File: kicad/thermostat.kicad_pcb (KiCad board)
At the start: 2 copper layers, 65 x 56 mm, 11 parts, among them P1 Conn_02x20_Odd_Even, U1 RELAY_HEAT

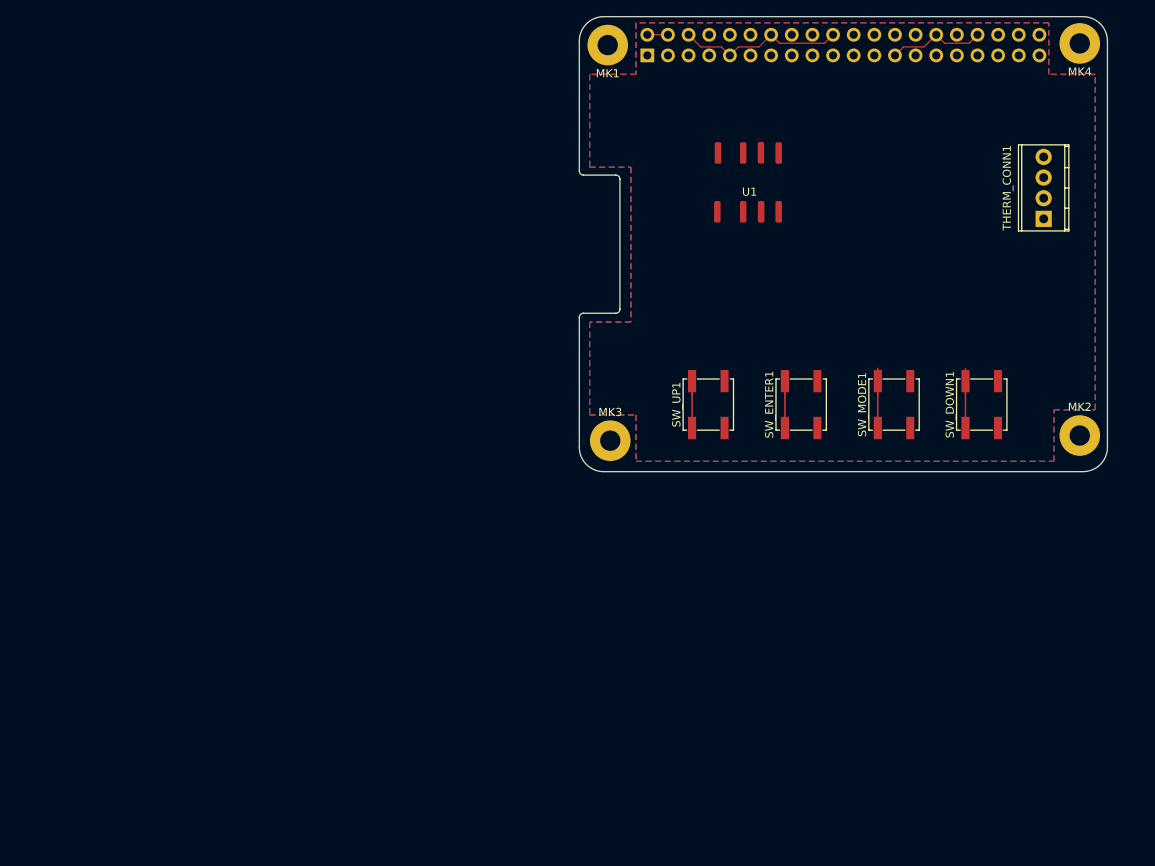
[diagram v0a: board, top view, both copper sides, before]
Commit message: First take at the bigger board
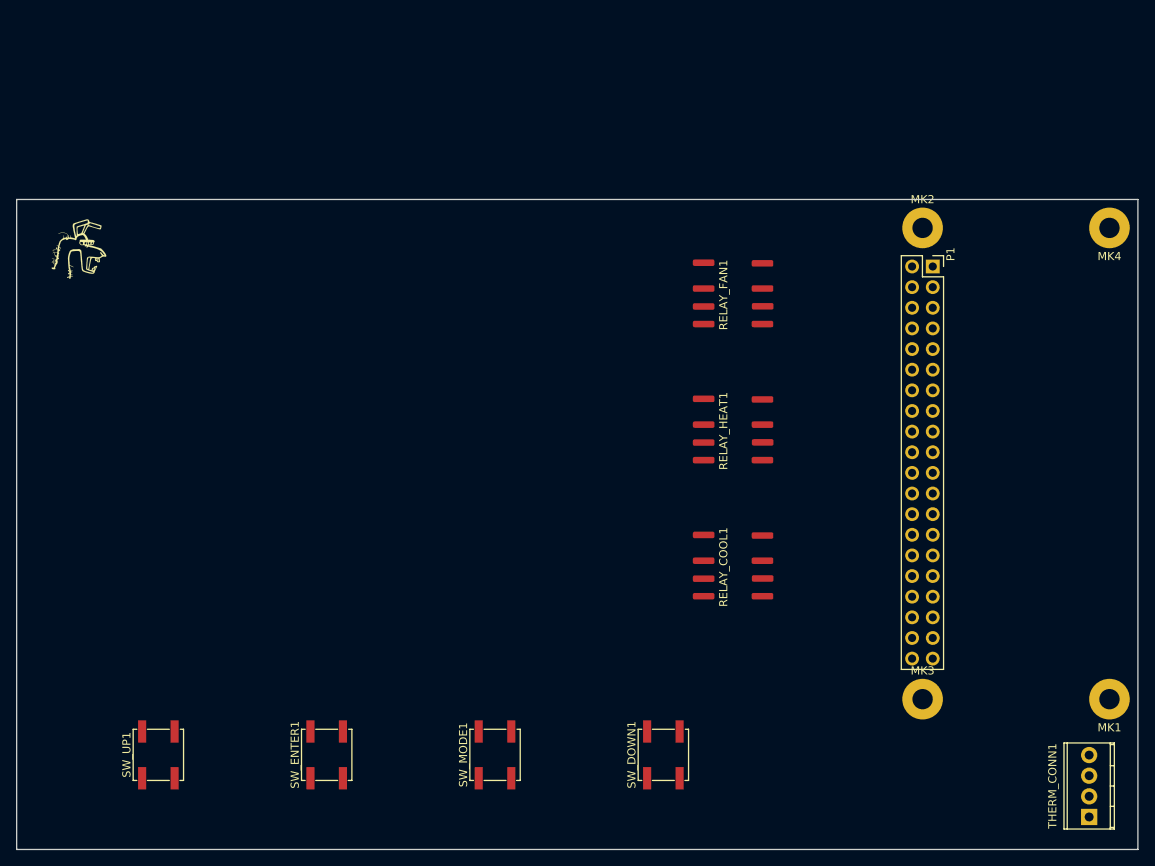
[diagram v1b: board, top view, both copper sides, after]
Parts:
- added G***: LOGO, project_footprints:LlamaHead, F.Cu at (138.5, 122.5)
- added RELAY_COOL1: RELAY_COOL, project_footprints:AGQ210A03, F.Cu at (218.2, 161.8)
- added RELAY_HEAT1: RELAY_HEAT, project_footprints:AGQ210A03, F.Cu at (218.2, 145.0)
- P1: moved to F.Cu
- RELAY_FAN1: renamed from U1; value RELAY_HEAT -> RELAY_FAN
- moved MK1 101.5 mm to (265.2, 178.0)
- moved SW_UP1 80.2 mm to (148.2, 184.9)
- moved THERM_CONN1 73.8 mm to (262.8, 192.5)
- moved SW_ENTER1 72.6 mm to (168.9, 184.9)
- moved SW_MODE1 65.3 mm to (189.6, 184.9)
- moved SW_DOWN1 58.3 mm to (210.3, 184.9)
- moved MK3 49.9 mm to (242.2, 178.0)
- moved P1 43.7 mm to (243.5, 124.8), turned to 0 degrees
- moved MK2 32.1 mm to (242.2, 120.0)
- moved MK4 23.0 mm to (265.2, 120.0)
- moved RELAY_FAN1 13.4 mm to (218.2, 128.2), turned to 270 degrees
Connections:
- P1 pad 33: (no net) -> /GPIO13(PWM1)
- P1 pad 35: (no net) -> /GPIO19(SPI1_MISO)
- RELAY_FAN1 pad 1: /GPIO6 -> /GPIO19(SPI1_MISO)
- RELAY_FAN1 pad 7: /HVAC_HEAT(WHITE) -> /HVAC_FAN(GREEN)
- THERM_CONN1 pad 3: (no net) -> /HVAC_COOL(YELLOW)
- THERM_CONN1 pad 4: (no net) -> /HVAC_FAN(GREEN)
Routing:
- net /GND: track 32.8 -> 0.00 mm
- net /GPIO21(SPI1_SCK): track 7.34 -> 0.00 mm
- net /GPIO16: track 7.34 -> 0.00 mm
- net /GPIO20(SPI1_MOSI): track 5.76 -> 0.00 mm
- net /GPIO12(PWM0): track 5.76 -> 0.00 mm
- net /PWR_5V: track 2.54 -> 0.00 mm
- removed copper zone on B.Cu, net /GND
- removed copper zone on F.Cu, net /PWR_3.3V
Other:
- board size 65 x 56 mm -> 138 x 80 mm
- board text added: "RaspberryPi Zero"
- board text removed: "DISPLAY"
